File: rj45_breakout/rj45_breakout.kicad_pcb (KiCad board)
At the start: 2 copper layers, 74.3 x 95.6 mm, 15 parts, among them J10 Conn_01x08, J6 RJ45_Shielded, J9 Conn_02x04_Odd_Even

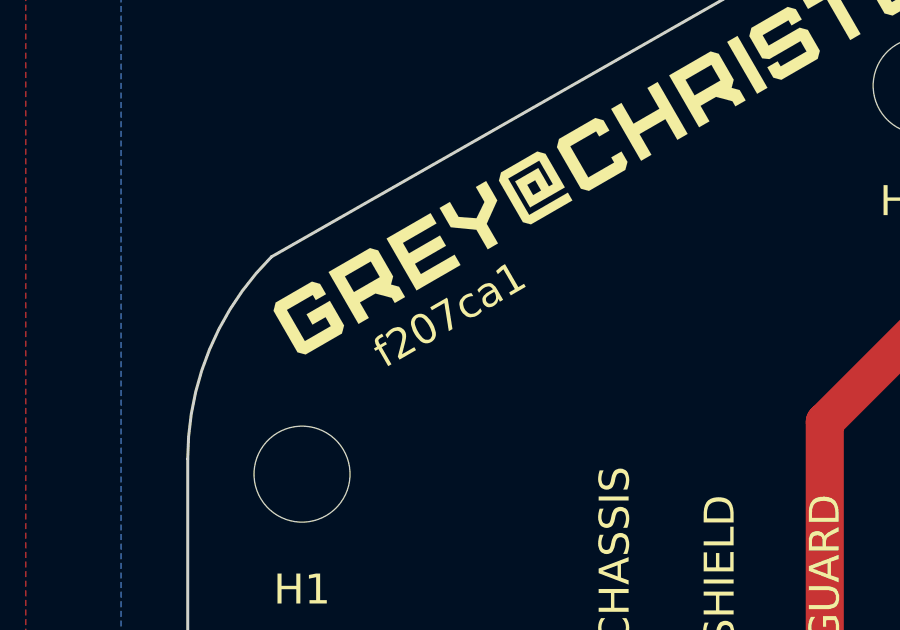
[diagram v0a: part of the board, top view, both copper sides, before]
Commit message: update silk
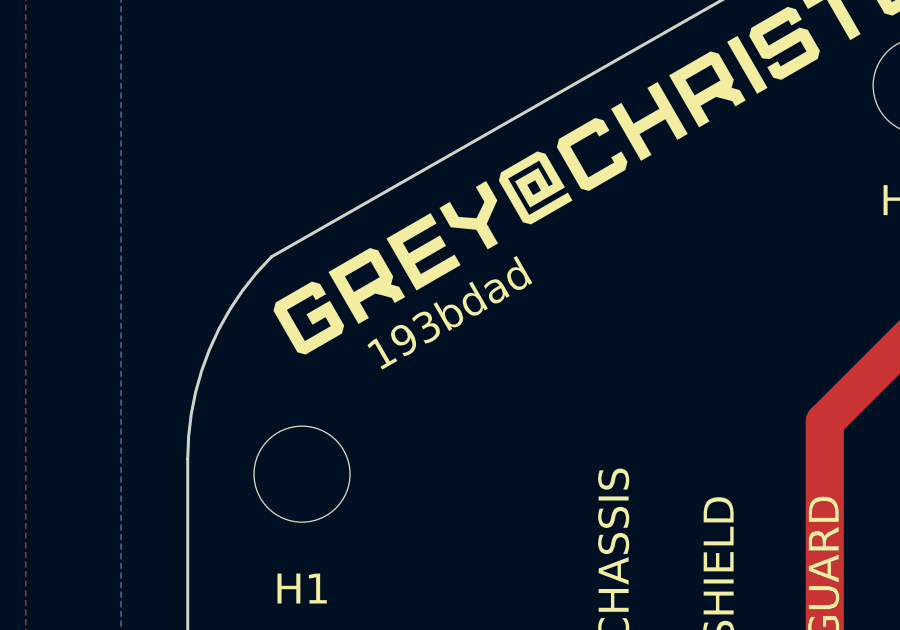
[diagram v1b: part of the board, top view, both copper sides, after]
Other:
- board text added: "193bdad"
- board text removed: "f207ca1"
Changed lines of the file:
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@@
     (effects (font (size 1 1) (thickness 0.15)) (justify right mirror))
   )
-  (gr_text "f207ca1" (at -30 -13.5 -150) (layer "B.SilkS")
+  (gr_text "193bdad" (at -30 -13.5 210) (layer "B.SilkS")
     (effects (font (size 1 1) (thickness 0.15)) (justify mirror))
   )
@@
     (effects (font (size 1 1) (thickness 0.15)) (justify left))
   )
-  (gr_text "f207ca1" (at -30 -13.5 30) (layer "F.SilkS")
+  (gr_text "193bdad" (at -30 -13.5 30) (layer "F.SilkS")
     (effects (font (size 1 1) (thickness 0.15)))
   )
